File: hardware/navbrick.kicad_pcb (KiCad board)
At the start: 2 copper layers, 110.7 x 52.3 mm, 93 parts, among them J50 Conn_01x06_Pin, J51 Conn_01x06_Pin, J52 USB4105-GF-A, J53 Conn_01x02_Pin, J54 Conn_01x02_Pin, J55 Conn_01x03_Pin, J56 Conn_01x03_Pin, J57 Conn_01x08_Pin, J58 Conn_01x08_Pin, Q1 DMP2004VK, Q2 DMP2004VK, Q3 DMP2004VK, Q4 DMP2004VK, SW50 PTS645SK50SMTR92, SW51 PTS645SK50SMTR92, U10 TLC59284, U11 TLC59284, U12 TLC59284, U13 TLC59284, U14 TLC59284, U15 TLC59284, U16 TLC59284, U2 MLX90393SLW-ABA-011, U3 MM74HCT540MTCX, U4 MS5611-01BA, U5 MM74HCT541MTCX, U50 CY7C65223D, U51 SAM-M10Q, U52 LTR-329ALS-01, U53 P3786E, U54 P3786E, U55 P3786E, U56 P3786E, U6 AVR128DA32x-xRXB, U7 FM25L16B, U8 LP2981A-33DBV, U9 TLC59284

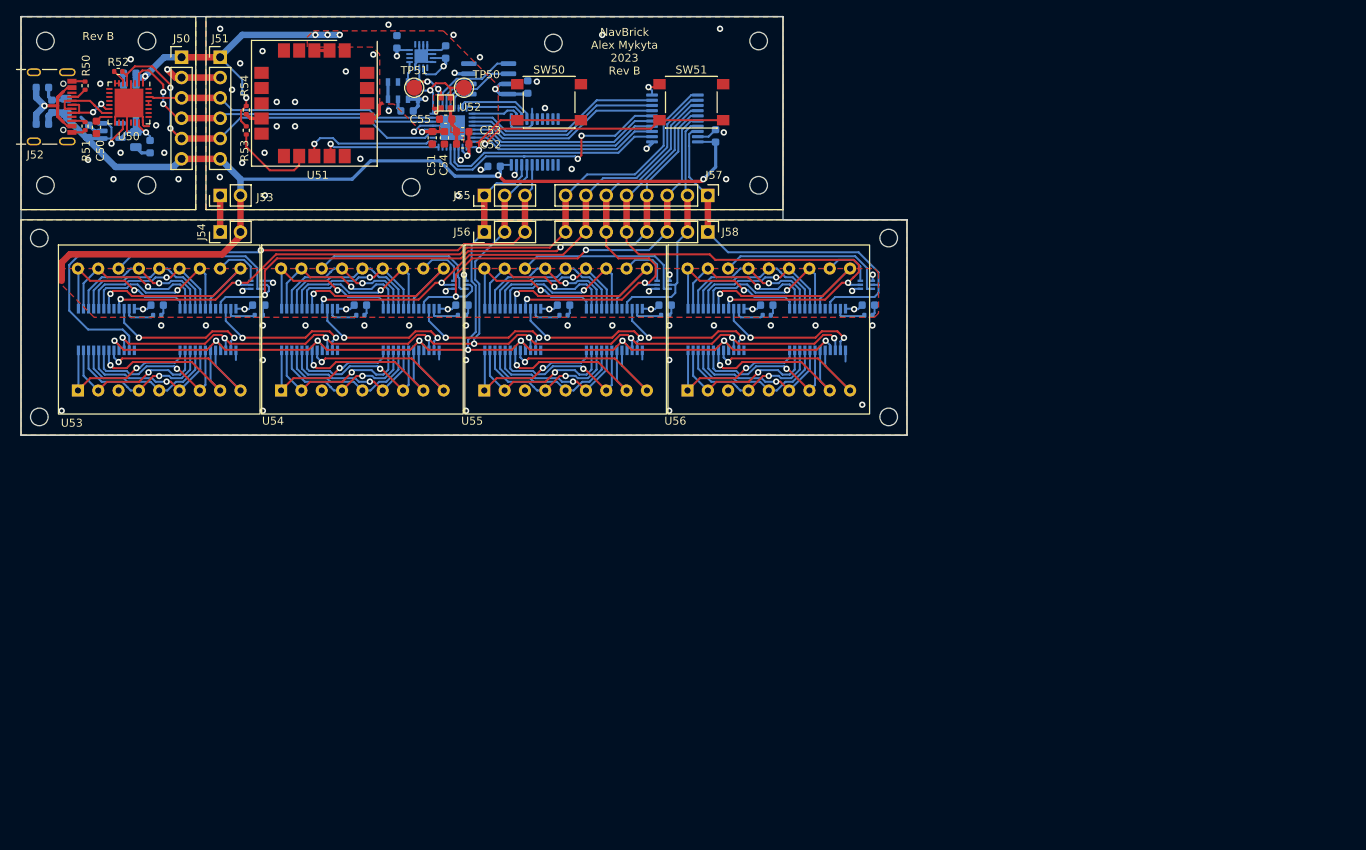
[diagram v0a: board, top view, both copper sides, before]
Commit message: Add pdf
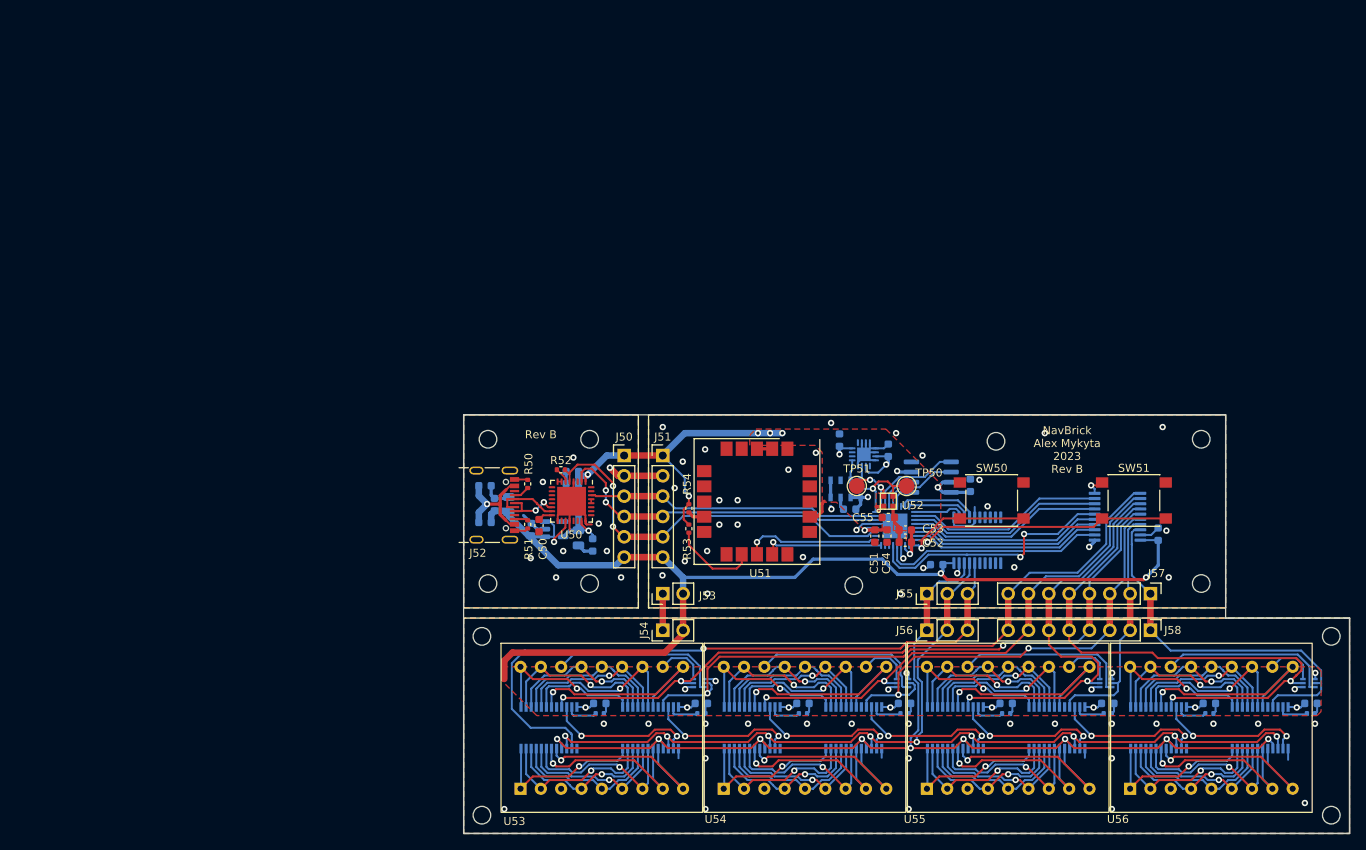
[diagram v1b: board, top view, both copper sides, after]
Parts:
- moved C50 74.4 mm to (9.38, 13.8)
- moved H56 74.4 mm to (15.7, 21.1)
- moved R50 74.4 mm to (7.96, 8.64)
- moved R51 74.4 mm to (7.96, 13.7)
- moved U10 74.4 mm to (86.8, 39.1)
- moved C10 74.4 mm to (13.5, 8.61)
- moved C11 74.4 mm to (2.62, 8.86)
- moved C12 74.4 mm to (5.59, 11.2)
- moved C13 74.4 mm to (3.82, 11.2)
- moved C14 74.4 mm to (8.43, 14.3)
- moved C15 74.4 mm to (59.1, 18.7)
- moved C16 74.4 mm to (105.9, 36.1)
- moved C17 74.4 mm to (93.2, 36.1)
- moved C18 74.4 mm to (80.5, 36.1)
- moved C19 74.4 mm to (67.8, 36.1)
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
